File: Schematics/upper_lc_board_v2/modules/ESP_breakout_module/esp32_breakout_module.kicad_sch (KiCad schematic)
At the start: 23 parts, among them J1 USB_C_Female_USB2_Small, SW1 SW_ESP_BOOT_MODE, SW2 SW_ESP_RESET, U1 ESP32-S3-WROOM-1-N16, U2 ISO1044BDR

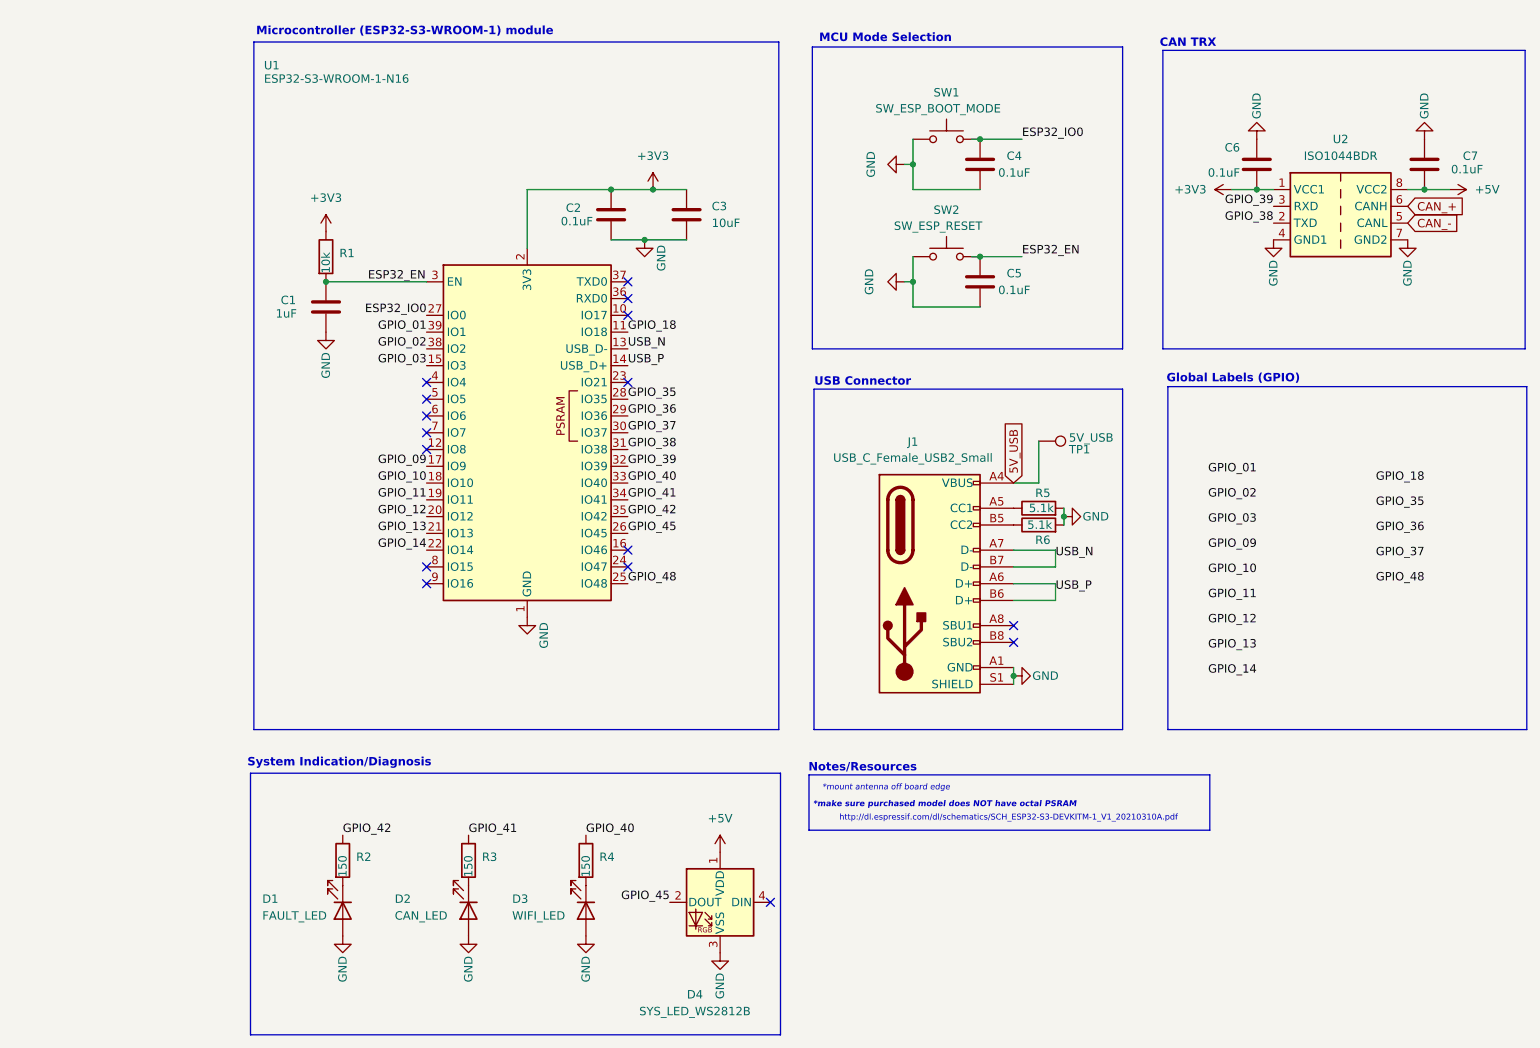
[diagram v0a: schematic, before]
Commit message: pcb design
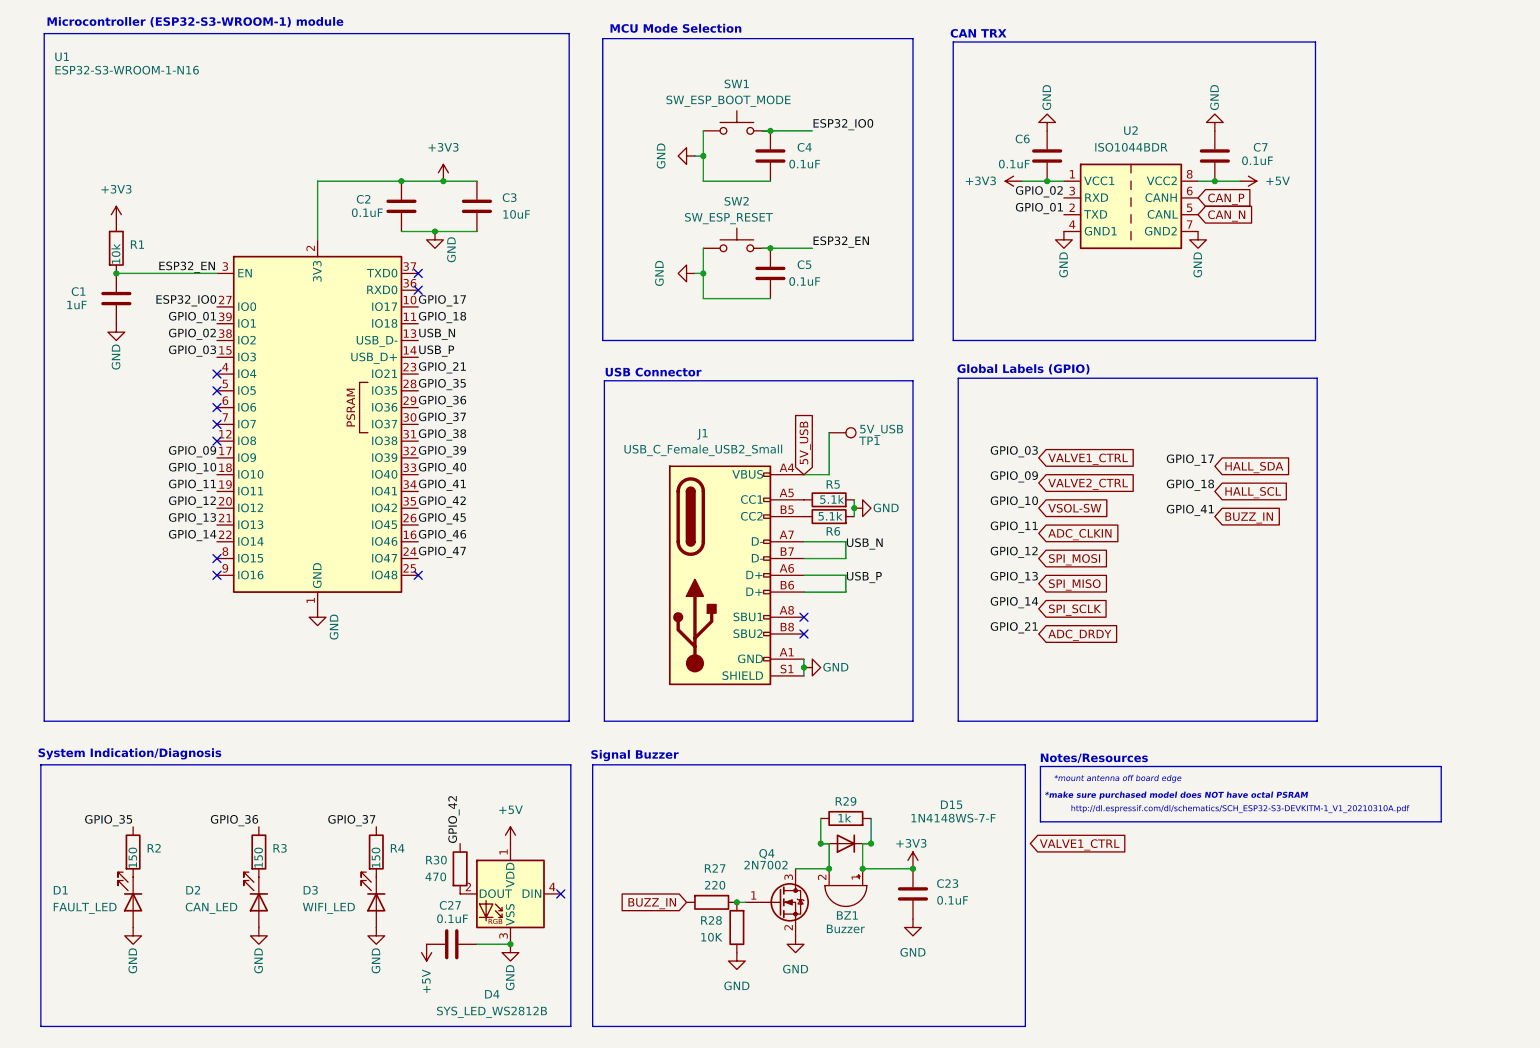
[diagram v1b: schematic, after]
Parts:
- added BZ1: Buzzer, Buzzer_Beeper:Buzzer_TDK_PS1240P02BT_D12.2mm_H6.5mm, symbol Device:Buzzer
- added C23, C27: 0.1uF, Capacitor_SMD:C_0603_1608Metric, symbol Device:C
- added D15: 1N4148WS-7-F, Diode_SMD:D_SOD-323, symbol Diode:1N4148WS
- added Q4: 2N7002, Package_TO_SOT_SMD:SOT-23, symbol Transistor_FET:2N7002
- added R27: 220, Resistor_SMD:R_0603_1608Metric, symbol Device:R
- added R28: 10K, Resistor_SMD:R_0603_1608Metric, symbol Device:R
- added R29: 1k, Resistor_SMD:R_0603_1608Metric, symbol Device:R
- added R30: 470, Resistor_SMD:R_0603_1608Metric, symbol Device:R
- J1: footprint USBC-CONN:USB_C_DB-108PWB -> Connector_USB:USB_C_Receptacle_GCT_USB4105-xx-A_16P_TopMnt_Horizontal
- U2: footprint ul_ISO1044BDR:SOIC_1044BDR_TEX -> ul_ISO1044BDR:SOIC127P600X175-8N
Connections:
- net +3V3: now also BZ1.1 (+), C23.1, D15.1 (K), R29.2
- net +5V: now also C27.1
- net GND: now also C23.2, C27.2, Q4.2 (S), R28.1
- net GPIO_01: now also U2.2 (TXD)
- net GPIO_02: now also U2.3 (RXD)
- net GPIO_35: now also R2.1
- net GPIO_36: now also R3.1
- net GPIO_37: now also R4.1
- net GPIO_38: no longer U2.2 (TXD)
- net GPIO_39: no longer U2.3 (RXD)
- net GPIO_40: no longer R4.1
- net GPIO_42: now also R30.1; no longer R2.1
- net GPIO_45: no longer D4.2 (DOUT)
- net HALL_SDA: now reaches U1.10 (IO17)
- net GPIO_46: now reaches U1.16 (IO46)
- net ADC_DRDY: now reaches U1.23 (IO21)
- net GPIO_47: now reaches U1.24 (IO47)
- net CAN_+ renamed CAN_P
- net CAN_- renamed CAN_N
- net GPIO_03 renamed VALVE1_CTRL
- net GPIO_09 renamed VALVE2_CTRL
- net GPIO_10 renamed VSOL-SW
- net GPIO_11 renamed ADC_CLKIN
- net GPIO_12 renamed SPI_MOSI
- net GPIO_13 renamed SPI_MISO
- net GPIO_14 renamed SPI_SCLK
- net GPIO_18 renamed HALL_SCL
- net GPIO_41 renamed BUZZ_IN
- net BUZZ_IN: now also R27.2; no longer R3.1
- net GPIO_48: no longer names the net of U1.25 (IO48)
- new net: Q4.1 (G), R27.1, R28.2
- new net: D4.2 (DOUT), R30.2
- new net: BZ1.2 (-), D15.2 (A), Q4.3 (D), R29.1
- no-connect marks 16 -> 13
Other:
- note added: "Signal Buzzer"
- moved on the sheet: C1, C2, C3, C4, C5, C6, C7, D1, D2, D3, D4, J1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
